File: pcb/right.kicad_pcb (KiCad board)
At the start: 2 copper layers, 135 x 95.7 mm, 51 parts, among them SW1 SW_PUSH, SW10 SW_PUSH, SW11 SW_PUSH, SW12 SW_PUSH, SW13 SW_PUSH, SW14 SW_PUSH, SW15 SW_PUSH, SW16 SW_PUSH, SW17 SW_PUSH, SW18 SW_PUSH, SW19 SW_PUSH, SW2 SW_PUSH, SW20 SW_PUSH, SW3 SW_PUSH, SW4 SW_PUSH, SW5 SW_PUSH, SW6 SW_PUSH, SW7 SW_PUSH, SW8 SW_PUSH, SW9 SW_PUSH

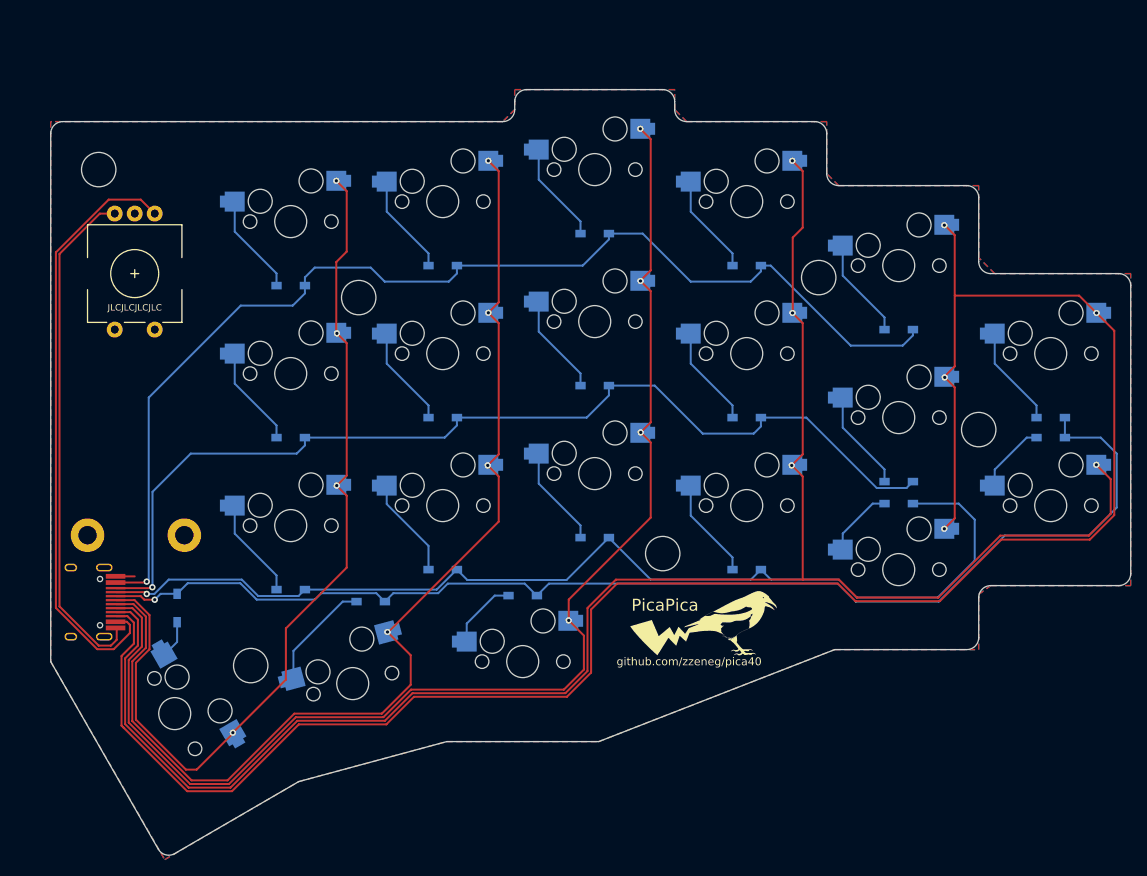
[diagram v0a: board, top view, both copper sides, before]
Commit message: v2
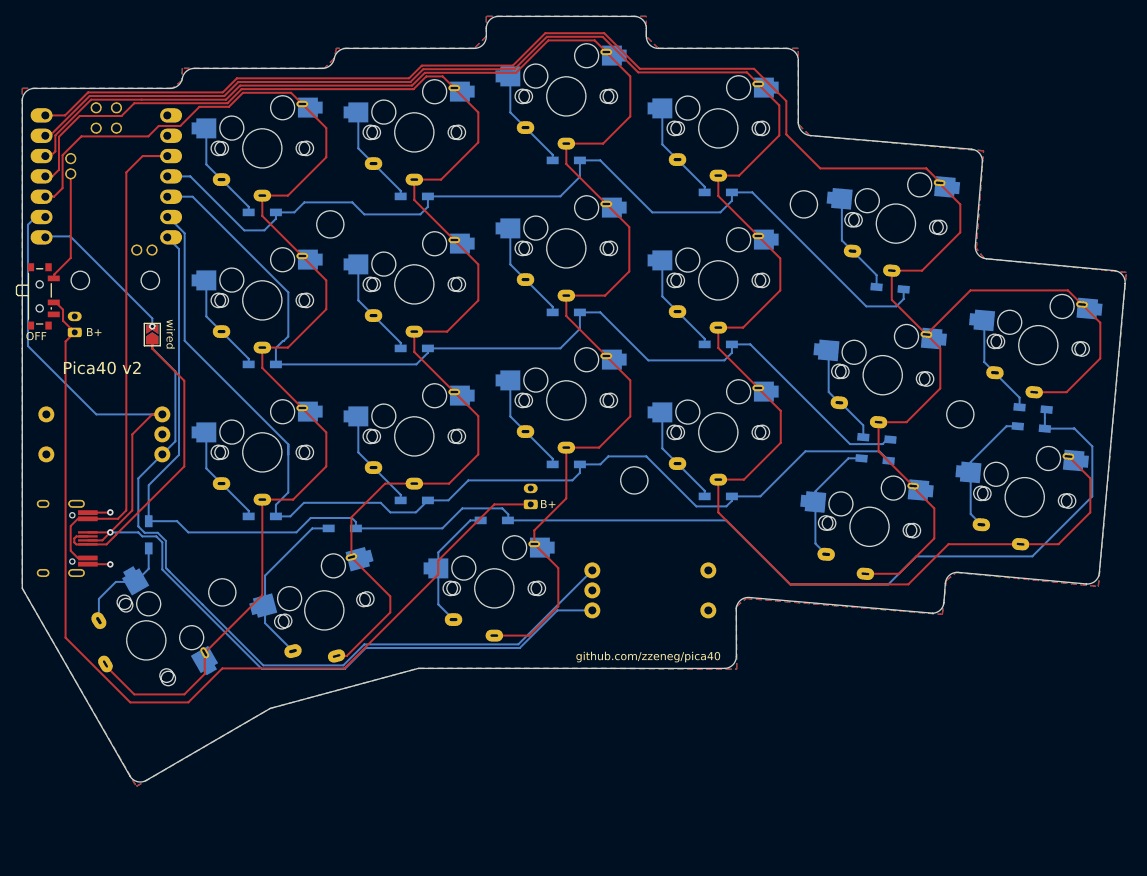
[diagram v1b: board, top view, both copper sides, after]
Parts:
- removed H8: MountingHole, kbd:M2_HOLE_v2
- added BATTCONN1: Conn_01x02_Female, pica:JST_PH_S2B-PH-K_1x02_P2.00mm, F.Cu at (88.0, 81.3)
- added BATTCONN2: Conn_01x02_Female, pica:JST_PH_S2B-PH-K_1x02_P2.00mm, F.Cu at (145.0, 102.8)
- added BATTSW1: SW_SPDT, Button_Switch_SMD:SW_SPDT_PCM12, F.Cu at (84.0, 76.8)
- added JP1: SolderJumper_2_Open, Jumper:SolderJumper-2_P1.3mm_Open_TrianglePad1.0x1.5mm, B.Cu at (97.7, 81.6)
- added JP2: SolderJumper_2_Open, Jumper:SolderJumper-2_P1.3mm_Open_TrianglePad1.0x1.5mm, F.Cu at (97.7, 81.6)
- added RE2: RotaryEncoder_Switch, pica:RotaryEncoder_EC11, F.Cu at (160.2, 113.6)
- added U1: xiao-ble, pica:xiao-ble-tht, F.Cu at (92.0, 61.9)
- G***: moved to B.Cu
- H1, H2, H3, H4, H5: footprint kbd:M2_HOLE_v2 -> pica:spacer_m2_3.4
- H6, H7: footprint kbd:M2_Hole_TH -> kbd:thread_m2
- SW1, SW10, SW11, SW12, SW13, SW14, SW15, SW16, SW17, SW18, SW19, SW2, SW3, SW4, SW5, SW6, SW7, SW8, SW9: footprint pica:CherryMX_Hotswap -> pica:CherryMX_Hotswap_ChocV2
- SW20: footprint pica:CherryMX_Hotswap_1.5 -> pica:CherryMX_Hotswap_ChocV2_1.5
- USB1: footprint typec:HRO-TYPE-C-31-M-12-HandSoldering -> pica:HRO-TYPE-C-31-M-12-data
- moved H6 32.1 mm to (97.5, 74.8)
- moved H7 31.9 mm to (88.7, 74.8)
- moved RE1 20.5 mm to (91.5, 94.1), turned to 180 degrees
- moved D18 10.0 mm to (140.4, 104.8)
- moved D12 9.81 mm to (168.4, 101.8)
- moved D13 9.81 mm to (149.4, 97.8)
- moved D7 9.81 mm to (168.4, 82.8)
- moved D8 9.81 mm to (149.4, 78.8)
- moved H4 9.81 mm to (157.9, 99.8)
- moved SW12 9.81 mm to (168.4, 93.8)
- moved SW13 9.81 mm to (149.4, 89.8)
- moved SW18 9.81 mm to (140.4, 113.3)
- moved SW7 9.81 mm to (168.4, 74.8)
- moved SW8 9.81 mm to (149.4, 70.8)
- moved D10 9.81 mm to (111.5, 85.3)
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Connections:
- D1 pad 1: row7 -> row0_r
- D10 pad 1: row6 -> row1_r
- D11 pad 1: row5 -> row2_r
- D12 pad 1: row5 -> row2_r
- D13 pad 1: row5 -> row2_r
- D14 pad 1: row5 -> row2_r
- D15 pad 1: row5 -> row2_r
- D16 pad 1: row4 -> row3_r
- D17 pad 1: row4 -> row3_r
- D18 pad 1: row4 -> row3_r
- D19 pad 1: row4 -> row3_r
- D2 pad 1: row7 -> row0_r
- D20 pad 1: row4 -> row3_r
- D3 pad 1: row7 -> row0_r
- D4 pad 1: row7 -> row0_r
- D5 pad 1: row7 -> row0_r
- D6 pad 1: row6 -> row1_r
- D7 pad 1: row6 -> row1_r
- D8 pad 1: row6 -> row1_r
- D9 pad 1: row6 -> row1_r
- RE1 pad A: ENCA -> ENCA_r
- RE1 pad B: ENCB -> ENCB_r
- RE1 pad C: GND -> GNDA
- RE1 pad S1: (no net) -> unconnected-(RE1-PadS1)
- RE1 pad S2: (no net) -> unconnected-(RE1-PadS2)
- SW1 pad 2: col0 -> col0_r
- SW10 pad 2: col4 -> col4_r
- SW11 pad 2: col0 -> col0_r
- SW12 pad 2: col1 -> col1_r
- SW13 pad 2: col2 -> col2_r
- SW14 pad 2: col3 -> col3_r
- SW15 pad 2: col4 -> col4_r
- SW16 pad 2: col0 -> col0_r
- SW17 pad 2: col1 -> col1_r
- SW18 pad 2: col2 -> col2_r
- SW19 pad 2: col3 -> col3_r
- SW2 pad 2: col1 -> col1_r
- SW20 pad 2: col4 -> col4_r
- SW3 pad 2: col2 -> col2_r
- SW4 pad 2: col3 -> col3_r
- SW5 pad 2: col4 -> col4_r
- SW6 pad 2: col0 -> col0_r
- SW7 pad 2: col1 -> col1_r
- SW8 pad 2: col2 -> col2_r
- SW9 pad 2: col3 -> col3_r
- USB1 pad 1: GND -> GNDA
- USB1 pad 11: ENCA -> VDD
- USB1 pad 12: ENCB -> GNDA
- USB1 pad 2: row7 -> VDD
- USB1 pad 5: row4 -> ENCB_r
- USB1 pad 6: col4 -> DATA_r
- USB1 pad 7: col3 -> ENCB_r
- USB1 pad 8: col2 -> DATA_r
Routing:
- net col0: track 249.3 -> 0.00 mm, vias 4 -> 0
- net col0_r: track 0.00 -> 238.8 mm
- net col1_r: track 0.00 -> 234.7 mm
- net col1: track 226.0 -> 0.00 mm, vias 4 -> 0
- net col2_r: track 0.00 -> 185.2 mm
- net row3_r: track 0.00 -> 183.7 mm
- net col3_r: track 0.00 -> 166.0 mm
- net col2: track 158.9 -> 0.00 mm, vias 4 -> 0
- net col4_r: track 0.00 -> 153.7 mm
- net row4: track 152.3 -> 0.00 mm, vias 1 -> 0
- net row7: track 143.8 -> 0.00 mm, vias 1 -> 0
- net col3: track 136.3 -> 0.00 mm, vias 4 -> 0
- net ENCB_r: track 0.00 -> 134.6 mm, vias 0 -> 1
- net row2_r: track 0.00 -> 133.2 mm
- net row5: track 132.9 -> 0.00 mm, vias 1 -> 0
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- added copper zone on B.Cu, net GNDA
- added copper zone on F.Cu, net GNDA
- removed copper zone on B.Cu, net GND
- removed copper zone on F.Cu, net GND
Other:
- board size 135 x 95.7 mm -> 137.8 x 95.7 mm
- board text added: "B+"
- board text added: "OFF"
- board text added: "Pica40 v2"
- board text added: "wired"
- board text added: "wireless"
- board text removed: "JLCJLCJLCJLC"
- board text removed: "PicaPica"
